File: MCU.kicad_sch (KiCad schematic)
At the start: 43 parts, among them J1 Conn_Coaxial, J6 USB_B, SW1 RotaryEncoder_Switch, SW2 RotaryEncoder_Switch, U1 FSA3157P6X, U10 FSA3157P6X, U11 FSA3157P6X, U12 FSA3157P6X, U14 AMS1117-3.3, U15 74HC14D653, U16 LM4040DBZ-3, U2 Screen, U8 STM32F103C8Tx, U9 CH340C

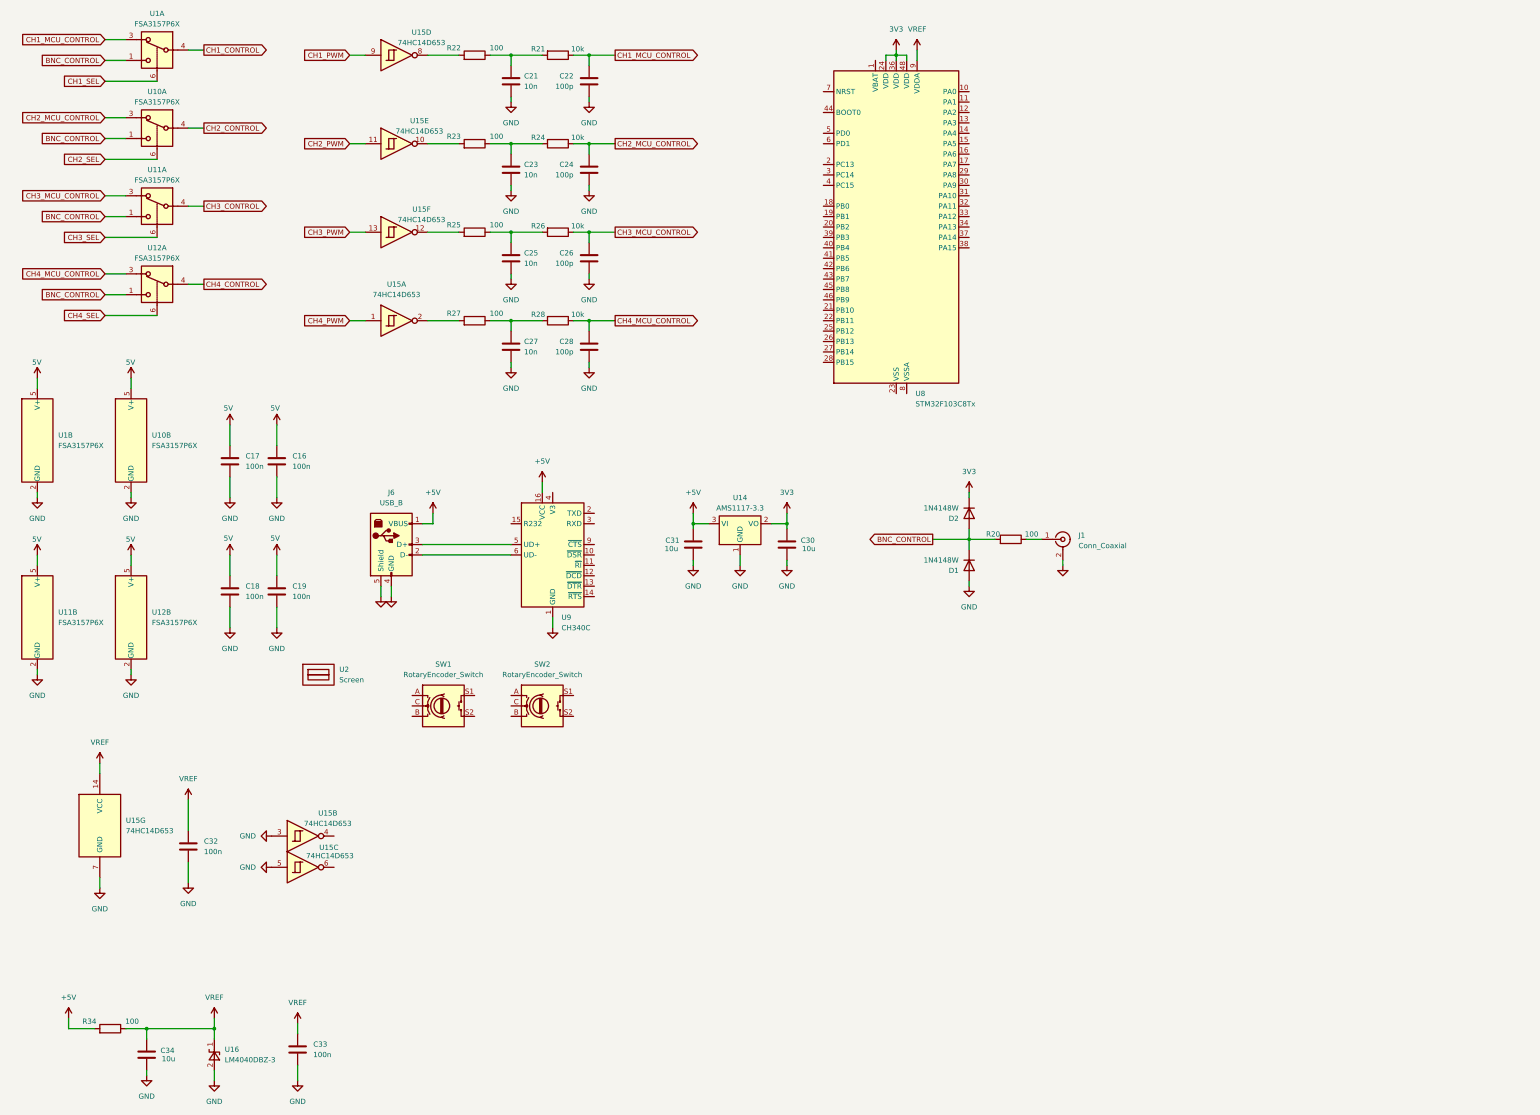
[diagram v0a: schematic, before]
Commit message: aesthetics.
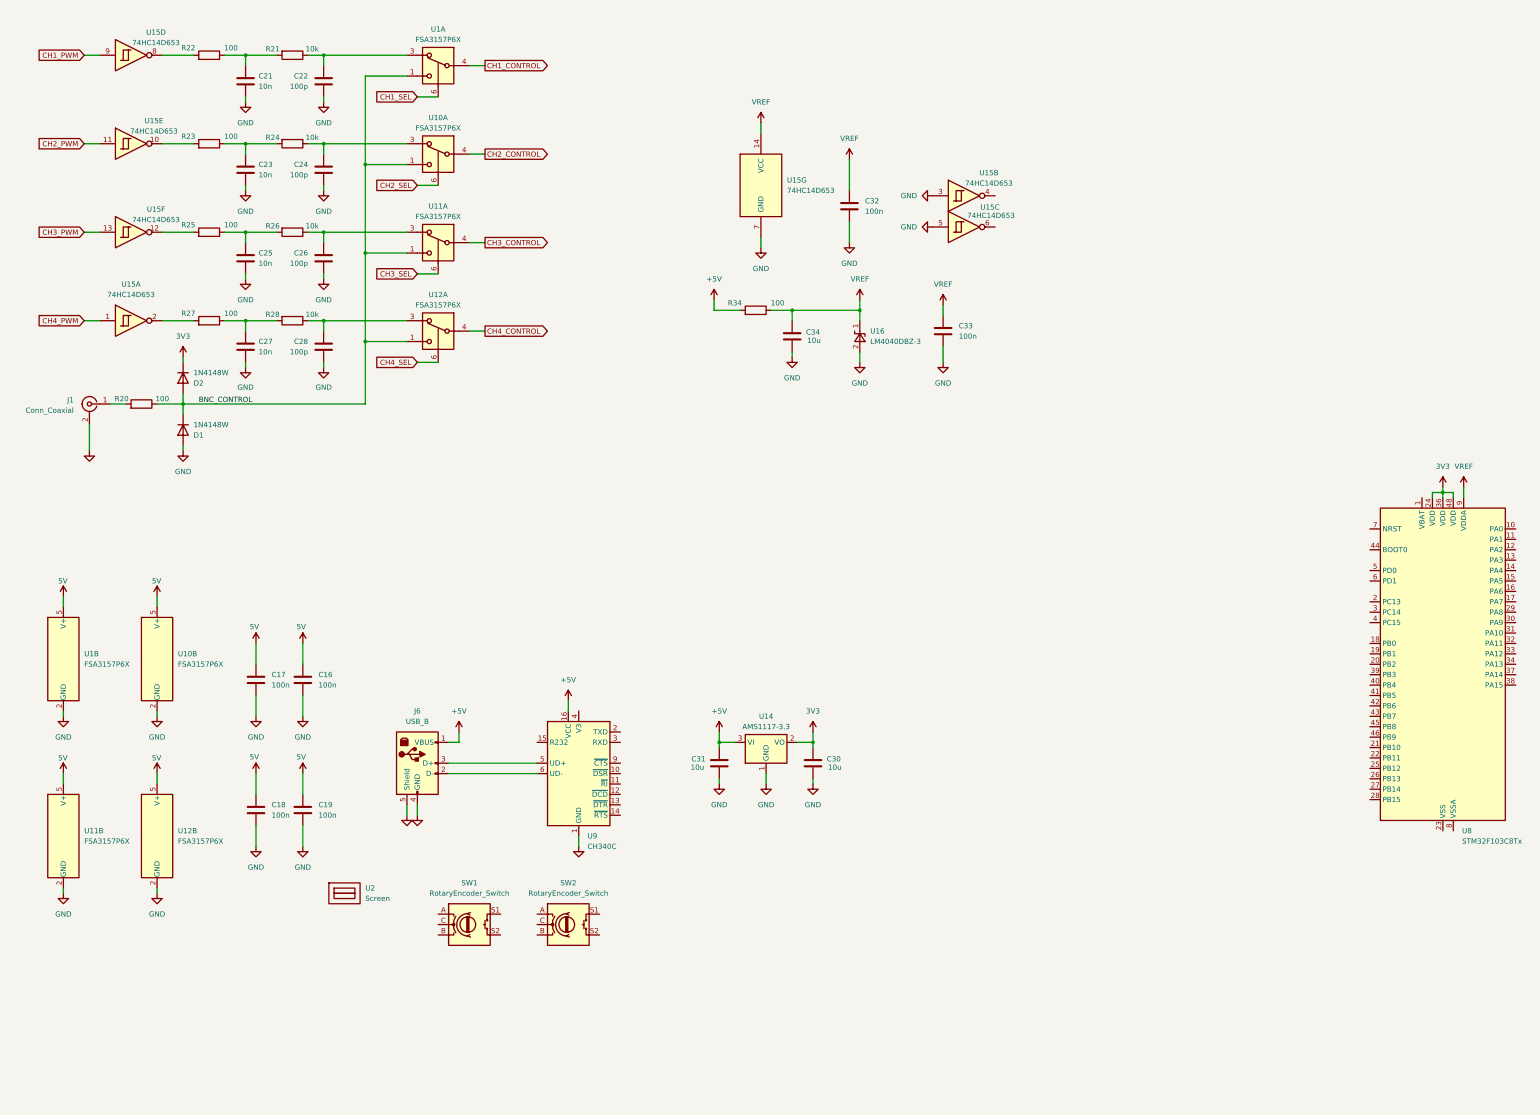
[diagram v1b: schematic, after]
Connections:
- net BNC_CONTROL: now also R20.1; no longer R20.2
- net at J1.1 (In): now also R20.2; no longer R20.1
- net CH1_MCU_CONTROL: no longer names the net of C22.2, R21.1, U1.3
- net CH2_MCU_CONTROL: no longer names the net of C24.2, R24.1, U10.3
- net CH3_MCU_CONTROL: no longer names the net of C26.2, R26.1, U11.3
- net CH4_MCU_CONTROL: no longer names the net of C28.2, R28.1, U12.3
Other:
- moved on the sheet: C16, C17, C18, C19, C21, C22, C23, C24, C25, C26, C27, C28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
